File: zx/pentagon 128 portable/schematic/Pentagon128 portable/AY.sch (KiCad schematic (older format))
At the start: 11 parts, among them U2 YM2149

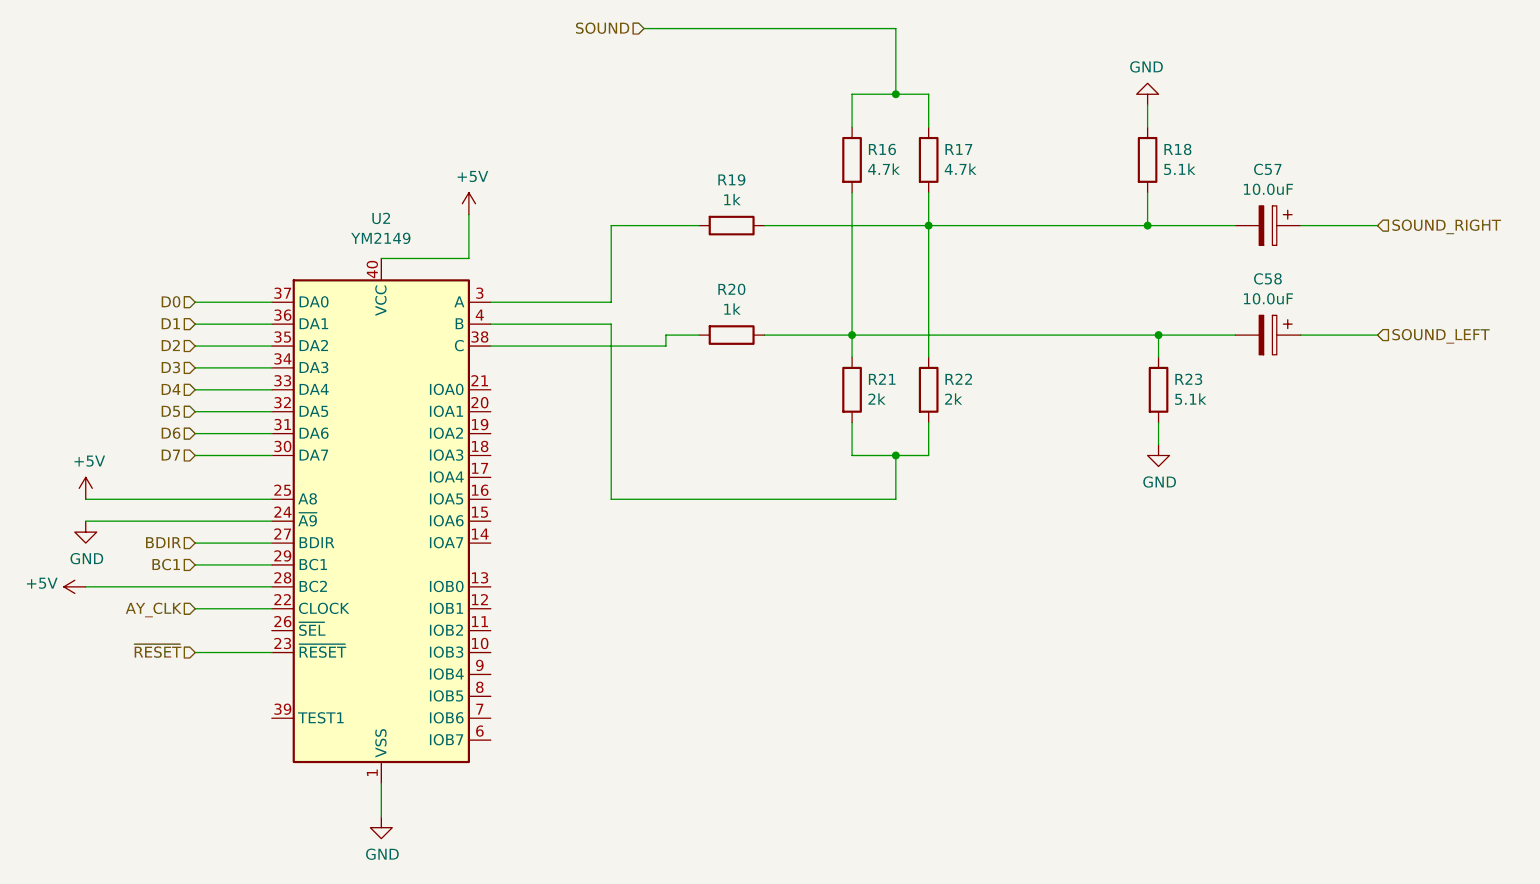
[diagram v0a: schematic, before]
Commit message: updated BOM
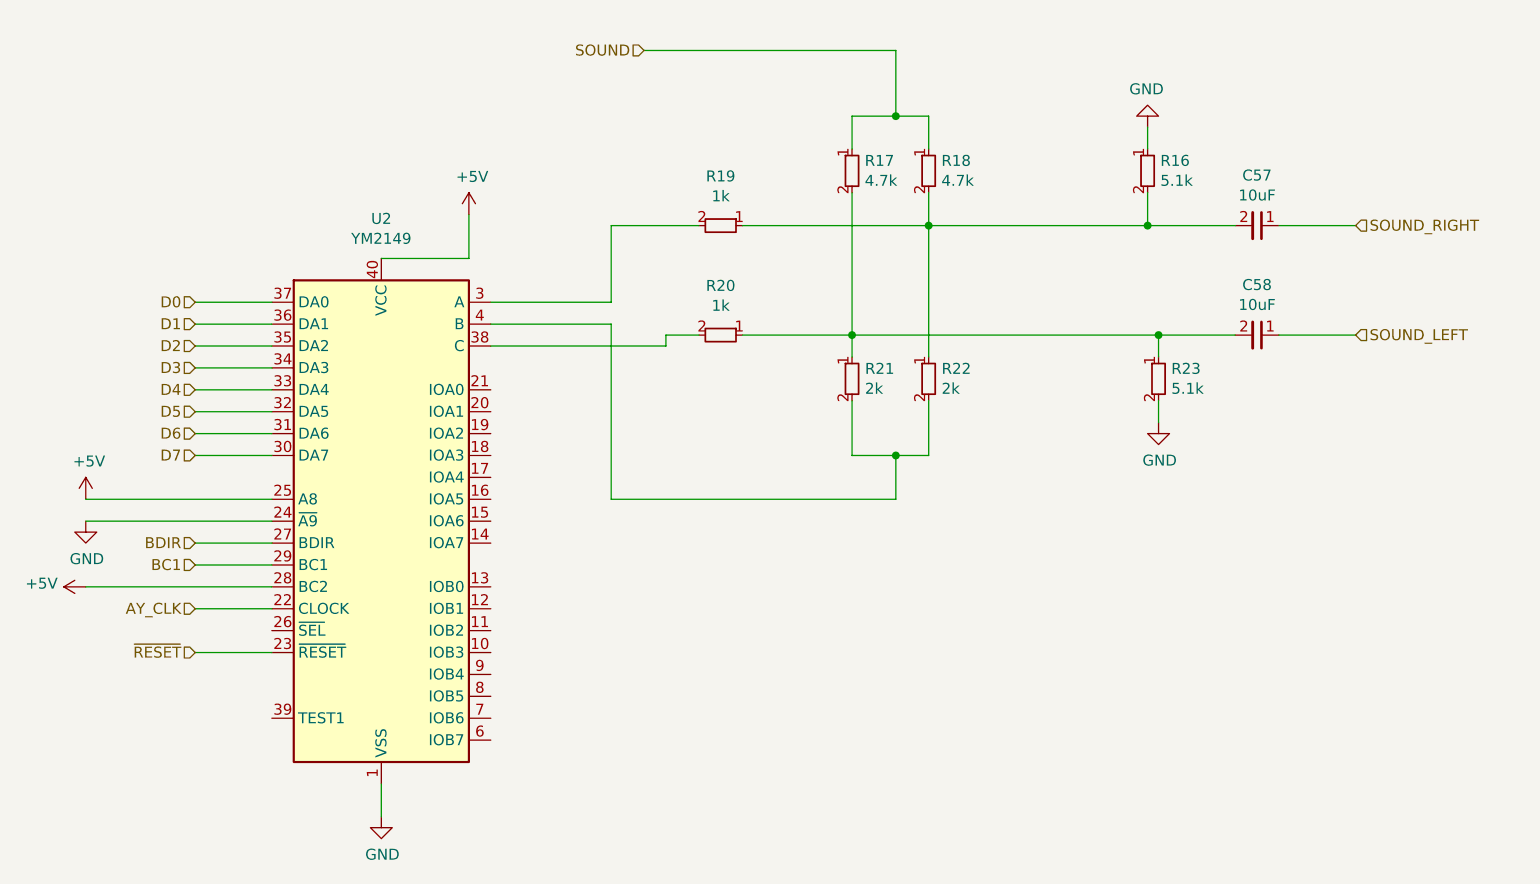
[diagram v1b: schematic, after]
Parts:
- removed C57, C58: 10.0uF, symbol Device:CP
- removed R16, R17: 4.7k, Resistor_SMD:R_0402_1005Metric, symbol Device:R
- removed R18, R23: 5.1k, Resistor_SMD:R_0402_1005Metric, symbol Device:R
- removed R19, R20: 1k, Resistor_SMD:R_0402_1005Metric, symbol Device:R
- removed R21, R22: 2k, Resistor_SMD:R_0402_1005Metric, symbol Device:R
- added C57, C58: 10uF, CAPC1005X55N, symbol SamacSys_Parts:10uF
- added R16, R23: 5.1k, RESC1005X40N, symbol SamacSys_Parts:5.1k
- added R17, R18: 4.7k, RESC1005X35N, symbol SamacSys_Parts:4.7k
- added R19, R20: 1k, RESC1005X35N, symbol SamacSys_Parts:1k
- added R21, R22: 2k, RESC1005X35N, symbol SamacSys_Parts:2k
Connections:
- net GND: now also R16.1, R23.2
- net SOUND: now also R17.1, R18.1
- net SOUND_LEFT: now also C58.1
- net SOUND_RIGHT: now also C57.1
- net at U2.3 (A): now also R19.2
- net at U2.38 (C): now also R20.2
- net at U2.4 (B): now also R21.2, R22.2
- new net: C57.2, R16.2, R18.2, R19.1, R22.1
- new net: C58.2, R17.2, R20.1, R21.1, R23.1
